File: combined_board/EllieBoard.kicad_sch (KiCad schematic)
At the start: 22 parts, among them J1 Flow Meter Conn, J10 Conn_01x06_Male, J11 Conn_01x04_Male, J12 Conn_01x04_Male, J13 Conn_01x06_Male, J14 Conn_01x06_Male, J15 Conn_01x04_Male, J16 Conn_01x04_Male, J17 Conn_01x06_Male, J18 Conn_01x06_Male, J19 Conn_01x04_Male, J2 Servo Conn 1, J20 Conn_01x04_Male, J3 Servo Conn 2, J4 Dean Conn, J5 Conn_01x06_Male, J6 Conn_01x06_Male, J7 Conn_01x04_Male, J8 Conn_01x04_Male, J9 Conn_01x06_Male

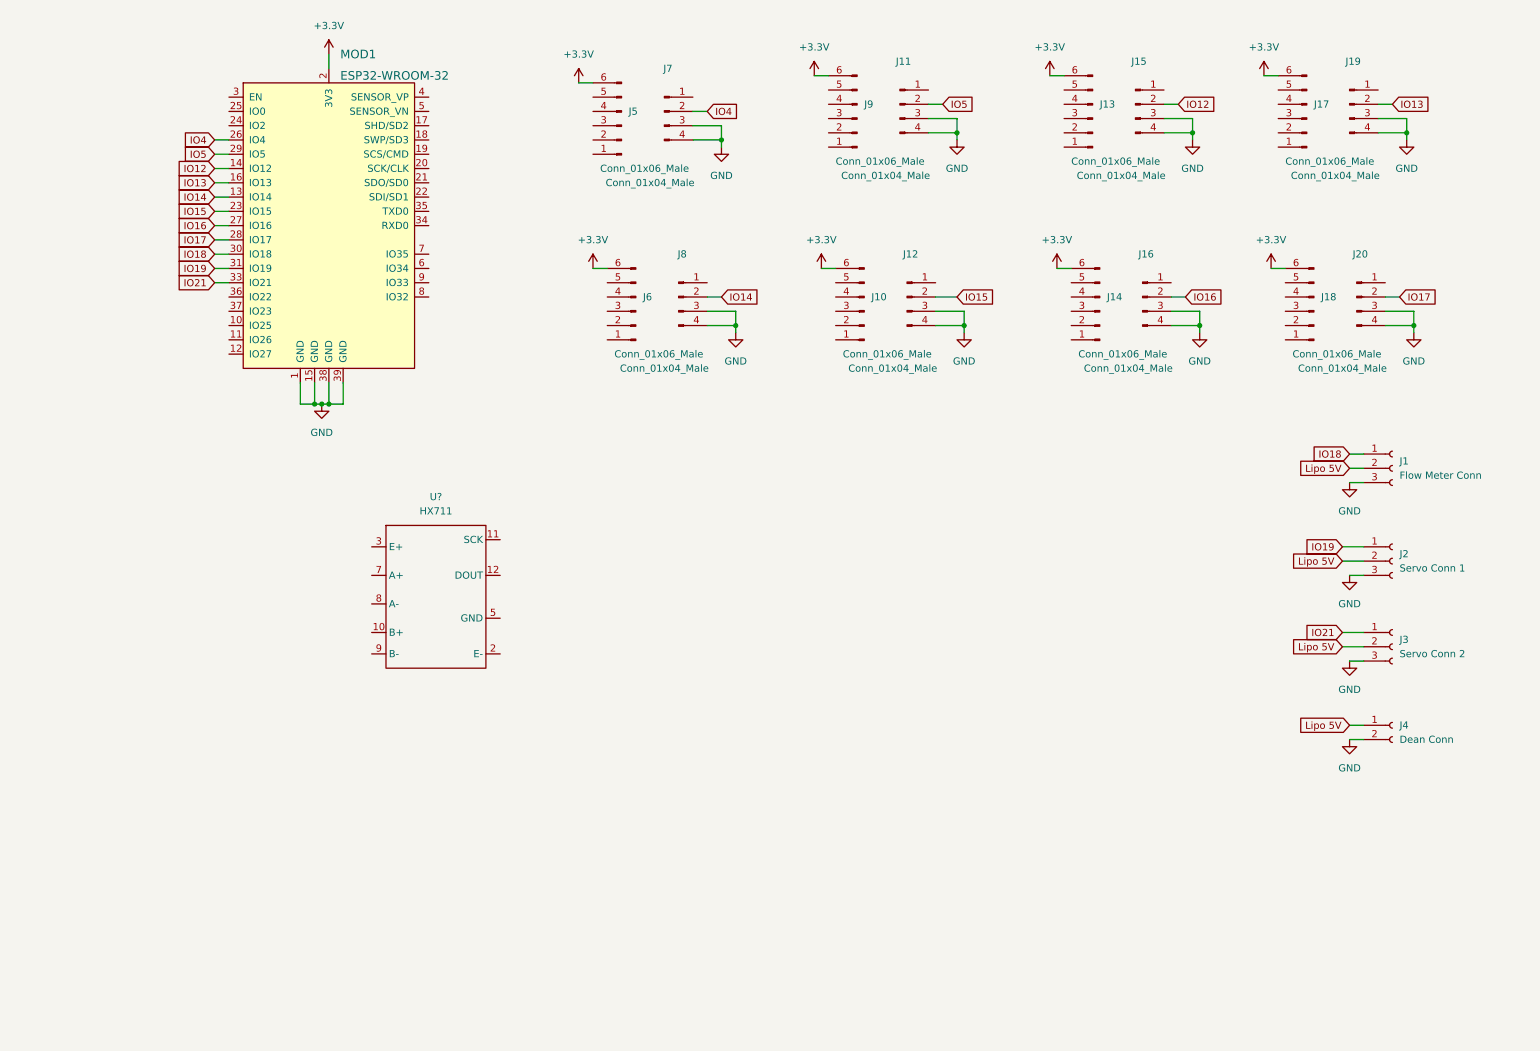
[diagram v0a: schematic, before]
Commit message: updated board electronics work session 04/04
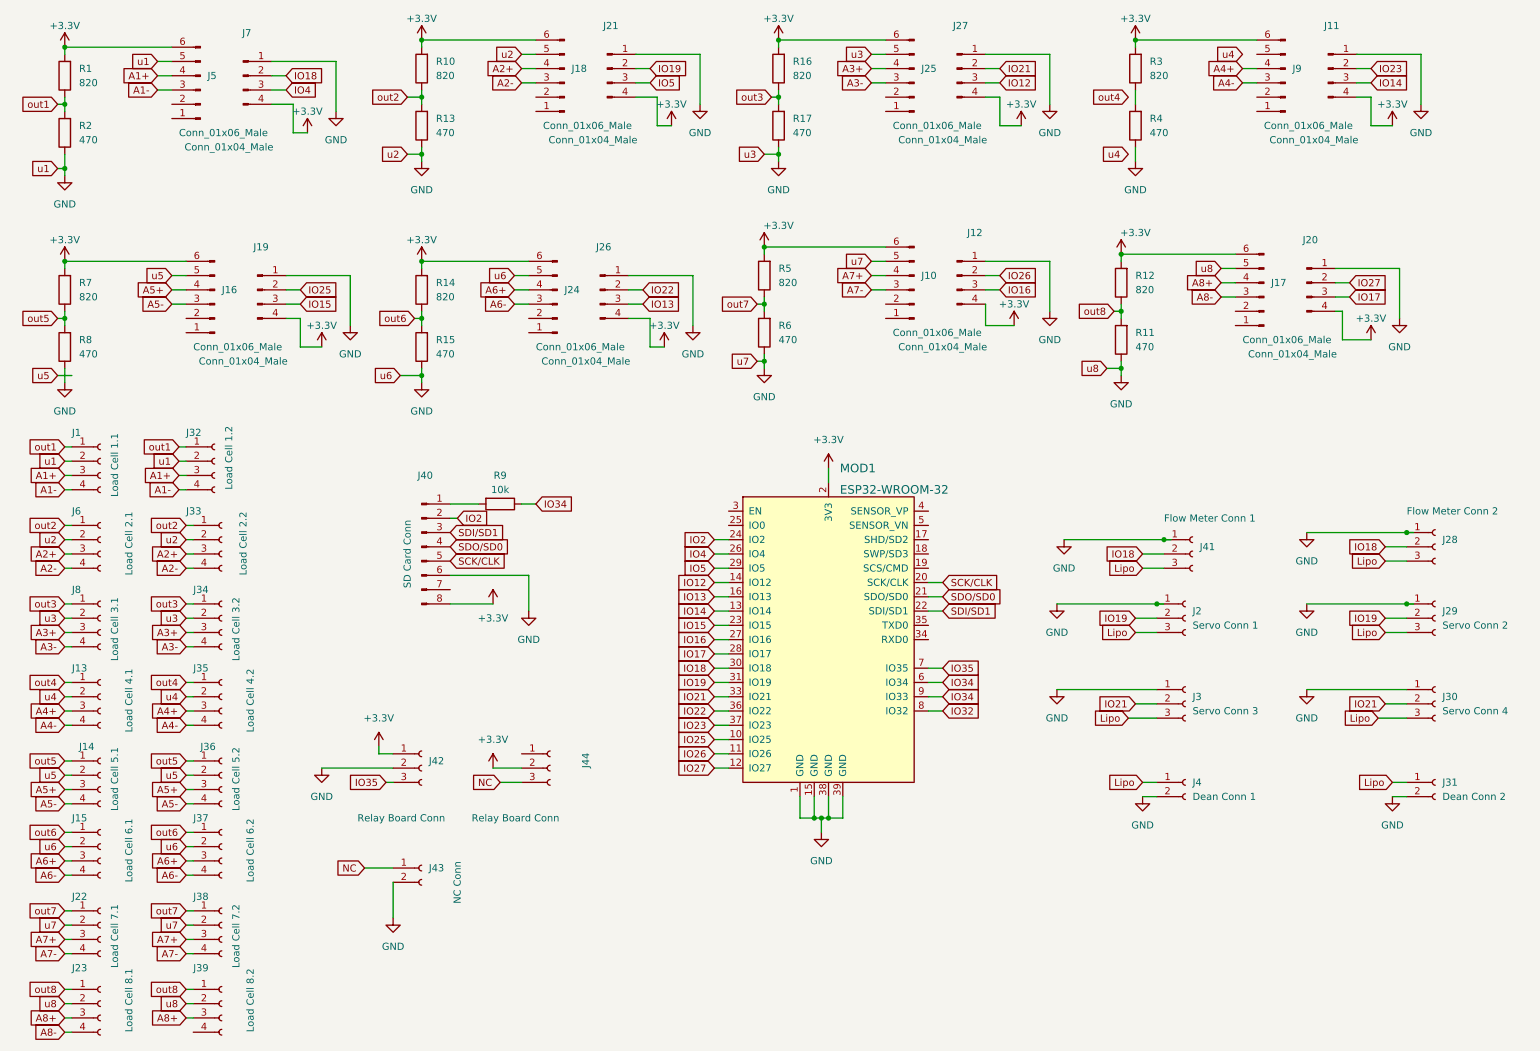
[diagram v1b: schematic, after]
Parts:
- removed J1: Flow Meter Conn, symbol Connector:Conn_01x03_Female
- removed J13, J14, J6: Conn_01x06_Male, symbol Connector:Conn_01x06_Male
- removed J15, J16, J8: Conn_01x04_Male, symbol Connector:Conn_01x04_Male
- removed U?: HX711, symbol hx711:HX711
- added J1: Load Cell 1.1, symbol Connector:Conn_01x04_Female
- added J13: Load Cell 4.1, symbol Connector:Conn_01x04_Female
- added J14: Load Cell 5.1, symbol Connector:Conn_01x04_Female
- added J15: Load Cell 6.1, symbol Connector:Conn_01x04_Female
- added J16, J24, J25: Conn_01x06_Male, symbol Connector:Conn_01x06_Male
- added J21, J26, J27: Conn_01x04_Male, symbol Connector:Conn_01x04_Male
- added J22: Load Cell 7.1, symbol Connector:Conn_01x04_Female
- added J23: Load Cell 8.1, symbol Connector:Conn_01x04_Female
- added J28: Flow Meter Conn 2, symbol Connector:Conn_01x03_Female
- added J29: Servo Conn 2, symbol Connector:Conn_01x03_Female
- added J30: Servo Conn 4, symbol Connector:Conn_01x03_Female
- added J31: Dean Conn 2, symbol Connector:Conn_01x02_Female
- added J32: Load Cell 1.2, symbol Connector:Conn_01x04_Female
- added J33: Load Cell 2.2, symbol Connector:Conn_01x04_Female
- added J34: Load Cell 3.2, symbol Connector:Conn_01x04_Female
- added J35: Load Cell 4.2, symbol Connector:Conn_01x04_Female
- added J36: Load Cell 5.2, symbol Connector:Conn_01x04_Female
- added J37: Load Cell 6.2, symbol Connector:Conn_01x04_Female
- added J38: Load Cell 7.2, symbol Connector:Conn_01x04_Female
- added J39: Load Cell 8.2, symbol Connector:Conn_01x04_Female
- added J40: SD Card Conn, symbol Connector:Conn_01x08_Male
- added J41: Flow Meter Conn 1, symbol Connector:Conn_01x03_Female
- added J42, J44: Relay Board Conn, symbol Connector:Conn_01x03_Female
- added J43: NC Conn, symbol Connector:Conn_01x02_Female
- added J6: Load Cell 2.1, symbol Connector:Conn_01x04_Female
- added J8: Load Cell 3.1, symbol Connector:Conn_01x04_Female
- added R1, R10, R12, R14, R16, R3, R5, R7: 820, Resistor_SMD:R_0201_0603Metric, symbol Device:R
- added R11, R13, R15, R17, R2, R4, R6, R8: 470, Resistor_SMD:R_0201_0603Metric, symbol Device:R
- added R9: 10k, Resistor_SMD:R_0201_0603Metric, symbol Device:R
- J3: value Servo Conn 2 -> Servo Conn 3
- J4: value Dean Conn -> Dean Conn 1
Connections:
- net +3V3: now also J11.4 (Pin_4), J12.4 (Pin_4), J19.4 (Pin_4), J20.4 (Pin_4), J7.4 (Pin_4), J16.6 (Pin_6), J21.4 (Pin_4), J24.6 (Pin_6), J25.6 (Pin_6), J26.4 (Pin_4), J27.4 (Pin_4), J40.8 (Pin_8), J42.1 (Pin_1), J44.2 (Pin_2), R1.2, R10.2, R12.2, R14.2, R16.2, R3.2, R5.2, R7.2
- net GND: now also J10.5 (Pin_5), J11.1 (Pin_1), J12.1 (Pin_1), J17.5 (Pin_5), J18.5 (Pin_5), J19.1 (Pin_1), J2.1 (Pin_1), J20.1 (Pin_1), J3.1 (Pin_1), J5.5 (Pin_5), J7.1 (Pin_1), J1.2 (Pin_2), J15.2 (Pin_2), J21.1 (Pin_1), J22.2 (Pin_2), J23.2 (Pin_2), J24.5 (Pin_5), J25.5 (Pin_5), J26.1 (Pin_1), J27.1 (Pin_1), J28.1 (Pin_1), J29.1 (Pin_1), J30.1 (Pin_1), J31.2 (Pin_2), J32.2 (Pin_2), J33.2 (Pin_2), J34.2 (Pin_2), J37.2 (Pin_2), J38.2 (Pin_2), J39.2 (Pin_2), J40.6 (Pin_6), J41.1 (Pin_1), J42.2 (Pin_2), J43.2 (Pin_2), J6.2 (Pin_2), J8.2 (Pin_2), R11.1, R13.1, R15.1, R17.1, R2.1, R4.1, R6.1, R8.1; no longer J11.3 (Pin_3), J11.4 (Pin_4), J12.3 (Pin_3), J12.4 (Pin_4), J19.3 (Pin_3), J19.4 (Pin_4), J2.3 (Pin_3), J20.3 (Pin_3), J20.4 (Pin_4), J3.3 (Pin_3), J7.3 (Pin_3), J7.4 (Pin_4)
- net IO12: now also J27.3 (Pin_3)
- net IO13: now also J26.3 (Pin_3); no longer J19.2 (Pin_2)
- net IO14: now also J11.3 (Pin_3)
- net IO15: now also J19.3 (Pin_3); no longer J12.2 (Pin_2)
- net IO16: now also J12.3 (Pin_3)
- net IO17: now also J20.3 (Pin_3); no longer J20.2 (Pin_2)
- net IO18: now also J7.2 (Pin_2), J28.2 (Pin_2), J41.2 (Pin_2)
- net IO19: now also J2.2 (Pin_2), J21.2 (Pin_2), J29.2 (Pin_2); no longer J2.1 (Pin_1)
- net IO21: now also J3.2 (Pin_2), J27.2 (Pin_2), J30.2 (Pin_2); no longer J3.1 (Pin_1)
- net IO4: now also J7.3 (Pin_3); no longer J7.2 (Pin_2)
- net IO5: now also J21.3 (Pin_3); no longer J11.2 (Pin_2)
- net A2-: now reaches J18.3 (Pin_3)
- net A2-: now also J33.4 (Pin_4), J6.4 (Pin_4)
- net A2+: now reaches J18.4 (Pin_4)
- net A2+: now also J33.3 (Pin_3), J6.3 (Pin_3)
- net A8-: now reaches J17.3 (Pin_3)
- net A8-: now also J23.4 (Pin_4)
- net A8+: now reaches J17.4 (Pin_4)
- net A8+: now also J23.3 (Pin_3), J39.3 (Pin_3)
- net IO25: now reaches MOD1.10 (IO25)
- net IO25: now also J19.2 (Pin_2)
- net IO26: now reaches MOD1.11 (IO26)
- net IO26: now also J12.2 (Pin_2)
- net IO27: now reaches MOD1.12 (IO27)
- net IO27: now also J20.2 (Pin_2)
- net SCK/CLK: now reaches MOD1.20 (SCK/CLK)
- net SCK/CLK: now also J40.5 (Pin_5)
- net SDO/SD0: now reaches MOD1.21 (SDO/SD0)
- net SDO/SD0: now also J40.4 (Pin_4)
- net SDI/SD1: now reaches MOD1.22 (SDI/SD1)
- net SDI/SD1: now also J40.3 (Pin_3)
- net IO2: now reaches MOD1.24 (IO2)
- net IO2: now also J40.2 (Pin_2)
- net IO22: now reaches MOD1.36 (IO22)
- net IO22: now also J26.2 (Pin_2)
- net IO23: now reaches MOD1.37 (IO23)
- net IO23: now also J11.2 (Pin_2)
- net IO34: now reaches MOD1.6 (IO34)
- net IO34: now also MOD1.9 (IO33), R9.1
- net IO35: now reaches MOD1.7 (IO35)
- net IO35: now also J42.3 (Pin_3)
- net IO32: now reaches MOD1.8 (IO32)
- net A7-: now reaches J10.3 (Pin_3)
- net A7-: now also J22.4 (Pin_4), J38.4 (Pin_4)
- net A7+: now reaches J10.4 (Pin_4)
- net A7+: now also J22.3 (Pin_3), J38.3 (Pin_3)
- net A4-: now reaches J9.3 (Pin_3)
- net A4-: now also J13.4 (Pin_4), J35.4 (Pin_4)
- net A4+: now reaches J9.4 (Pin_4)
- net A4+: now also J13.3 (Pin_3), J35.3 (Pin_3)
- net A1-: now reaches J5.3 (Pin_3)
- net A1-: now also J1.4 (Pin_4), J32.4 (Pin_4)
- net A1+: now reaches J5.4 (Pin_4)
- net A1+: now also J1.3 (Pin_3), J32.3 (Pin_3)
- removed net Lipo 5V: J2.2 (Pin_2), J3.2 (Pin_2), J4.1 (Pin_1)
- new net: R3.1, R4.2
- new net: J40.1 (Pin_1), R9.2
- new net A3+: J25.4 (Pin_4), J34.3 (Pin_3), J8.3 (Pin_3)
- new net A3-: J25.3 (Pin_3), J34.4 (Pin_4), J8.4 (Pin_4)
- new net A5+: J14.3 (Pin_3), J16.4 (Pin_4), J36.3 (Pin_3)
- new net A5-: J14.4 (Pin_4), J16.3 (Pin_3), J36.4 (Pin_4)
- new net A6+: J15.3 (Pin_3), J24.4 (Pin_4), J37.3 (Pin_3)
- new net A6-: J15.4 (Pin_4), J24.3 (Pin_3), J37.4 (Pin_4)
- new net Lipo: J2.3 (Pin_3), J29.3 (Pin_3), J3.3 (Pin_3), J30.3 (Pin_3), J4.1 (Pin_1), J41.3 (Pin_3)
- new net Lipo : J28.3 (Pin_3), J31.1 (Pin_1)
- new net NC: J43.1 (Pin_1), J44.3 (Pin_3)
- new net out1: J1.1 (Pin_1), J32.1 (Pin_1), R1.1, R2.2
- new net out2: J33.1 (Pin_1), J6.1 (Pin_1), R10.1, R13.2
- new net out3: J34.1 (Pin_1), J8.1 (Pin_1), R16.1, R17.2
- new net out4: J13.1 (Pin_1), J35.1 (Pin_1)
- new net out5: J14.1 (Pin_1), J36.1 (Pin_1), R7.1, R8.2
- new net out6: J15.1 (Pin_1), J37.1 (Pin_1), R14.1, R15.2
- new net out7: J22.1 (Pin_1), J38.1 (Pin_1), R5.1, R6.2
- new net out8: J23.1 (Pin_1), J39.1 (Pin_1), R11.2, R12.1
- new net u4: J13.2 (Pin_2), J35.2 (Pin_2)
- new net u5: J14.2 (Pin_2), J16.5 (Pin_5), J36.2 (Pin_2)
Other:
- moved on the sheet: J2, J3, J4, J5, J7, MOD1
